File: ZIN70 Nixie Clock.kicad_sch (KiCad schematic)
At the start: 34 parts, among them Q1 PN2222A, Q2 PN2222A, Q3 PN2222A, Q4 PN2222A, U1 HV5122, U2 HV5122, U3 OKI-78SR-3.3_1.5-W36-C, U4 OKI-78SR-3.3_1.5-W36-C

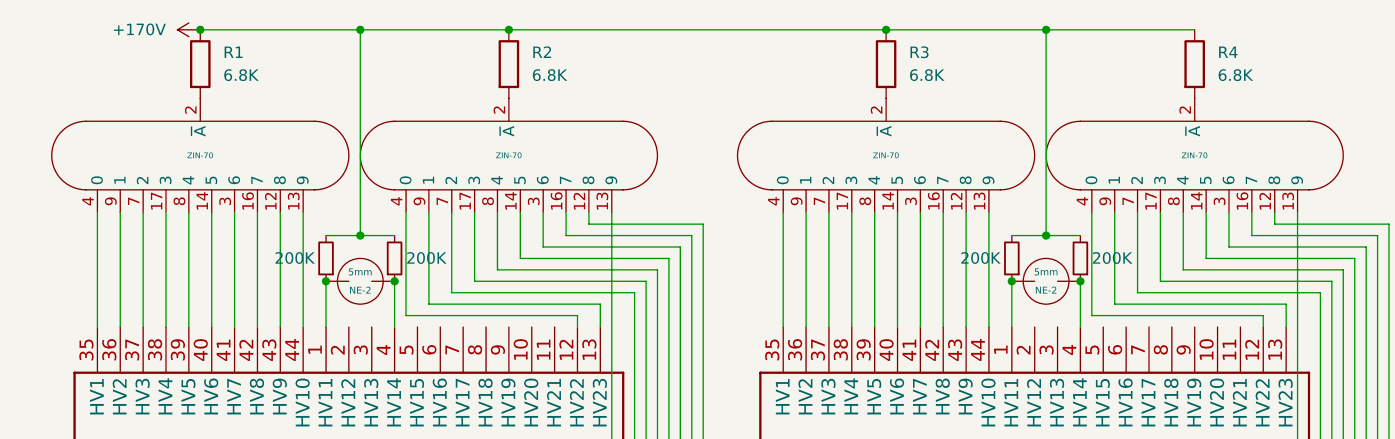
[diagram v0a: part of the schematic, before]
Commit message: Adjustments I forgot to save
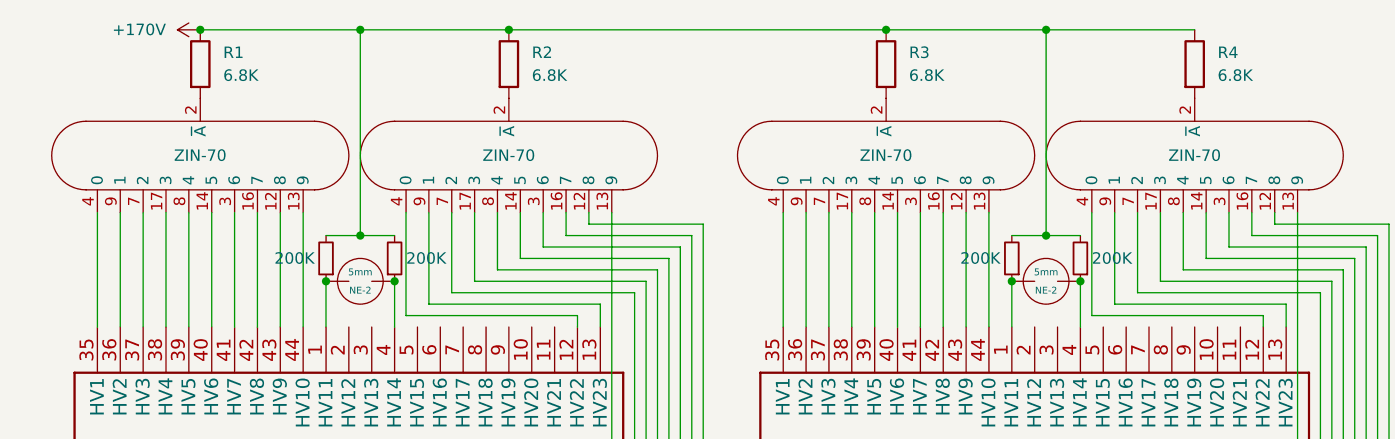
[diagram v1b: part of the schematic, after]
